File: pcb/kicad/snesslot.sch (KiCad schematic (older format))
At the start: 5 parts, among them J1 SNESCART_EXT, U1 74ALVC164245, U2 74ALVC164245, U3 74ALVC164245, U5 74LVC1T45

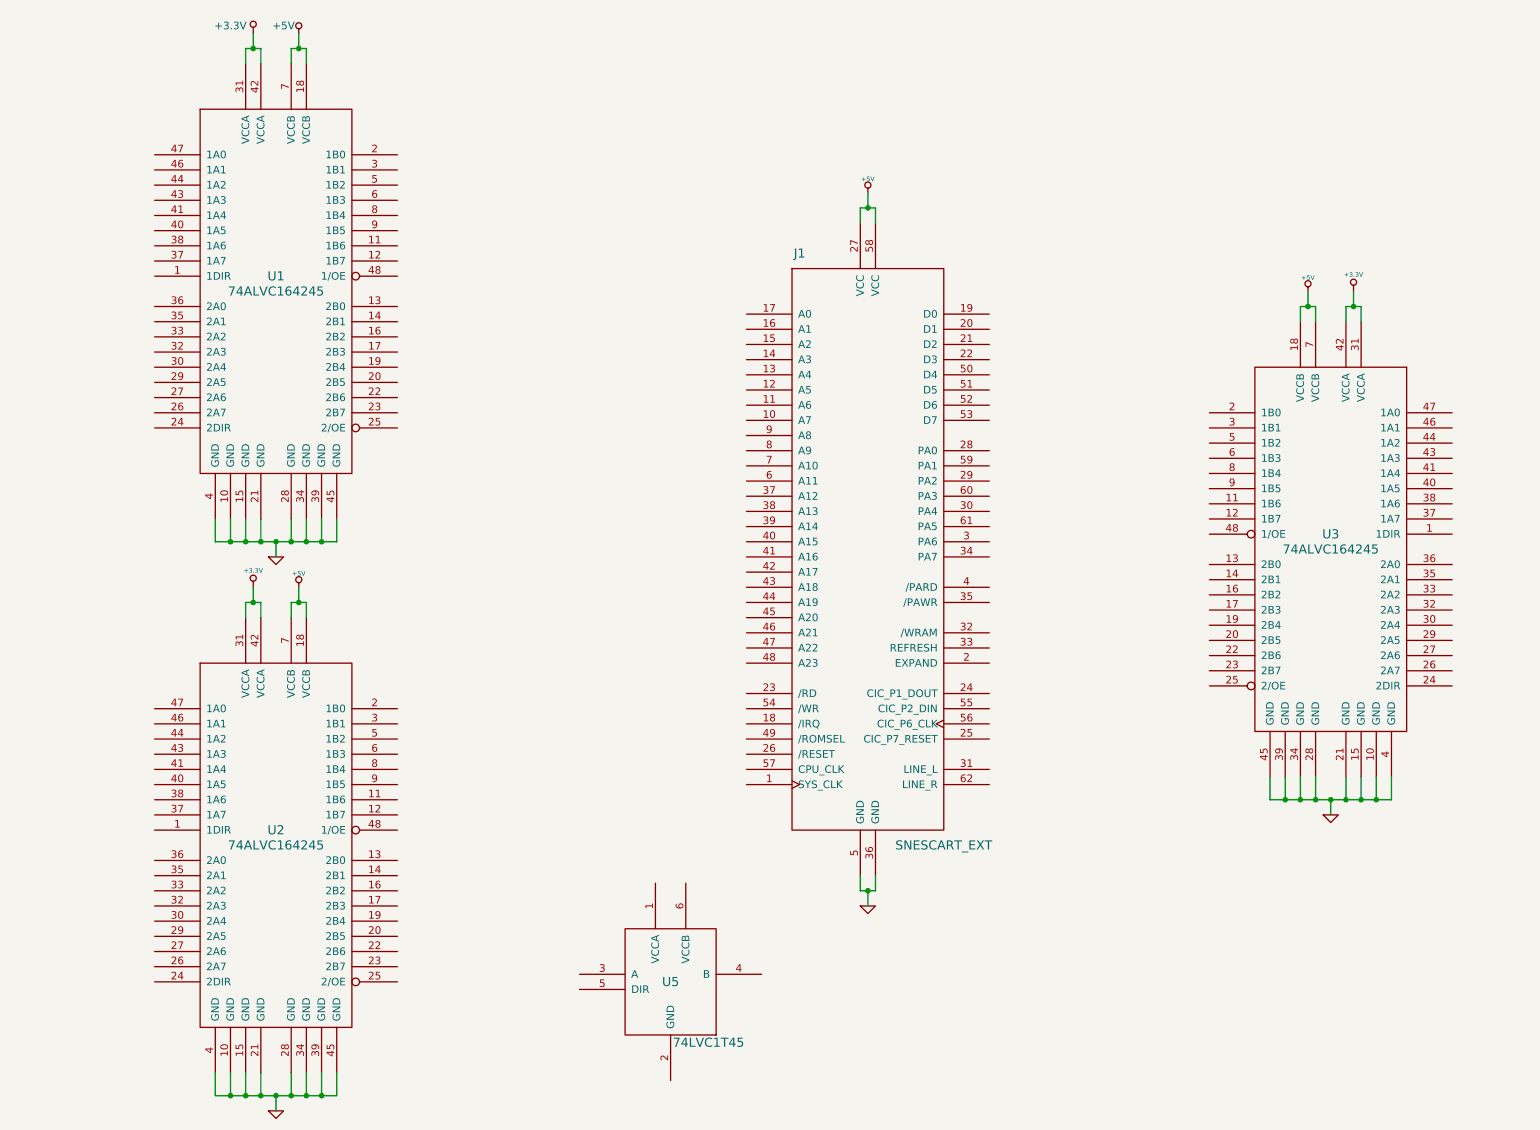
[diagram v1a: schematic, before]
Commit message: kicad wip
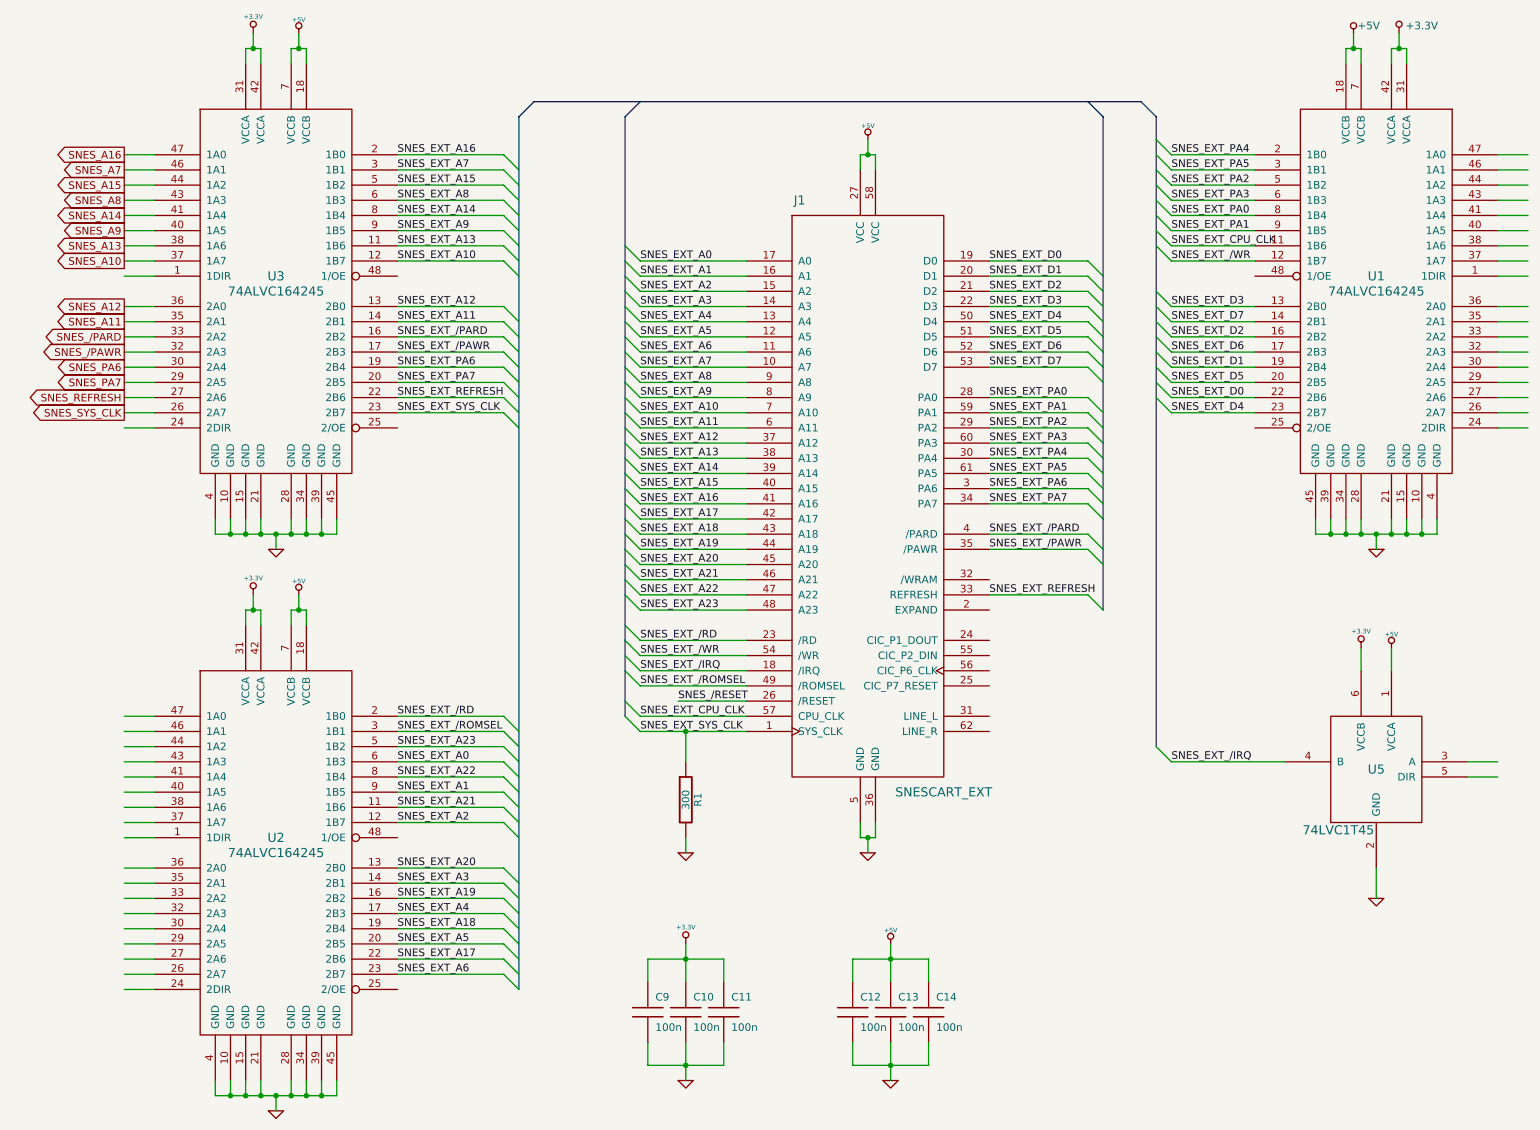
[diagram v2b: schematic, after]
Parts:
- added C10, C11, C12, C13, C14, C9: 100n, symbol C
- added R1: 300, symbol R
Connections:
- net labels added: SNES_/PARD, SNES_/PAWR, SNES_/RESET, SNES_A10, SNES_A11, SNES_A12, SNES_A13, SNES_A14, SNES_A15, SNES_A16, SNES_A7, SNES_A8, SNES_A9, SNES_EXT_/IRQ, SNES_EXT_/PARD, SNES_EXT_/PAWR, SNES_EXT_/RD, SNES_EXT_/ROMSEL, SNES_EXT_/WR, SNES_EXT_A0, SNES_EXT_A1, SNES_EXT_A10, SNES_EXT_A11, SNES_EXT_A12, SNES_EXT_A13, SNES_EXT_A14, SNES_EXT_A15, SNES_EXT_A16, SNES_EXT_A17, SNES_EXT_A18, SNES_EXT_A19, SNES_EXT_A2, SNES_EXT_A20, SNES_EXT_A21, SNES_EXT_A22, SNES_EXT_A23, SNES_EXT_A3, SNES_EXT_A4, SNES_EXT_A5, SNES_EXT_A6, SNES_EXT_A7, SNES_EXT_A8, SNES_EXT_A9, SNES_EXT_CPU_CLK, SNES_EXT_D0, SNES_EXT_D1, SNES_EXT_D2, SNES_EXT_D3, SNES_EXT_D4, SNES_EXT_D5, SNES_EXT_D6, SNES_EXT_D7, SNES_EXT_PA0, SNES_EXT_PA1, SNES_EXT_PA2, SNES_EXT_PA3, SNES_EXT_PA4, SNES_EXT_PA5, SNES_EXT_PA6, SNES_EXT_PA7, SNES_EXT_REFRESH, SNES_EXT_SYS_CLK, SNES_PA6, SNES_PA7, SNES_REFRESH, SNES_SYS_CLK
- wire segments 62 -> 238
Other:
- moved on the sheet: J1, U1, U2, U3, U5
